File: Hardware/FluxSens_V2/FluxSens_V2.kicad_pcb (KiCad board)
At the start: 2 copper layers, 35 parts, among them J1 Conn_01x08, U1 HMC1051Z, U2 RC4558, U3 MAX662ACSA+

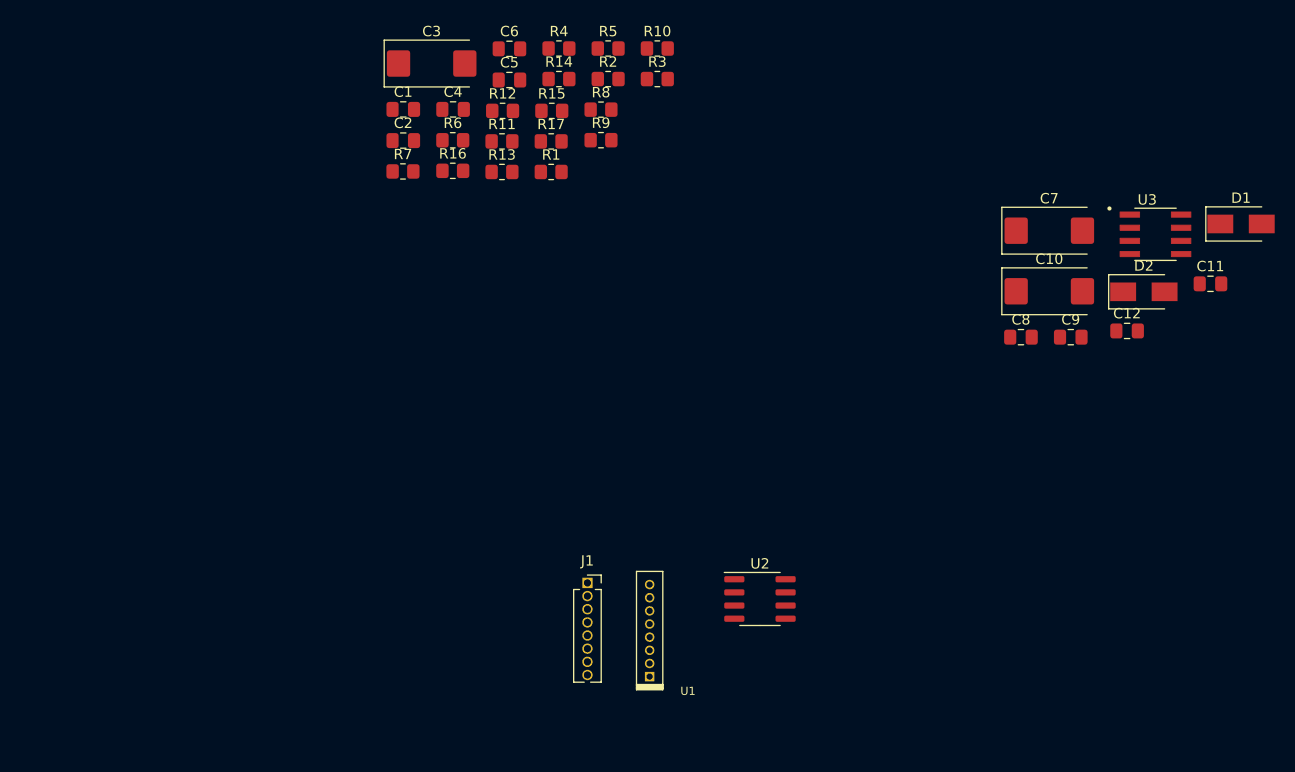
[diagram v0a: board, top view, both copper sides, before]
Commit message: finished the V2 board layout
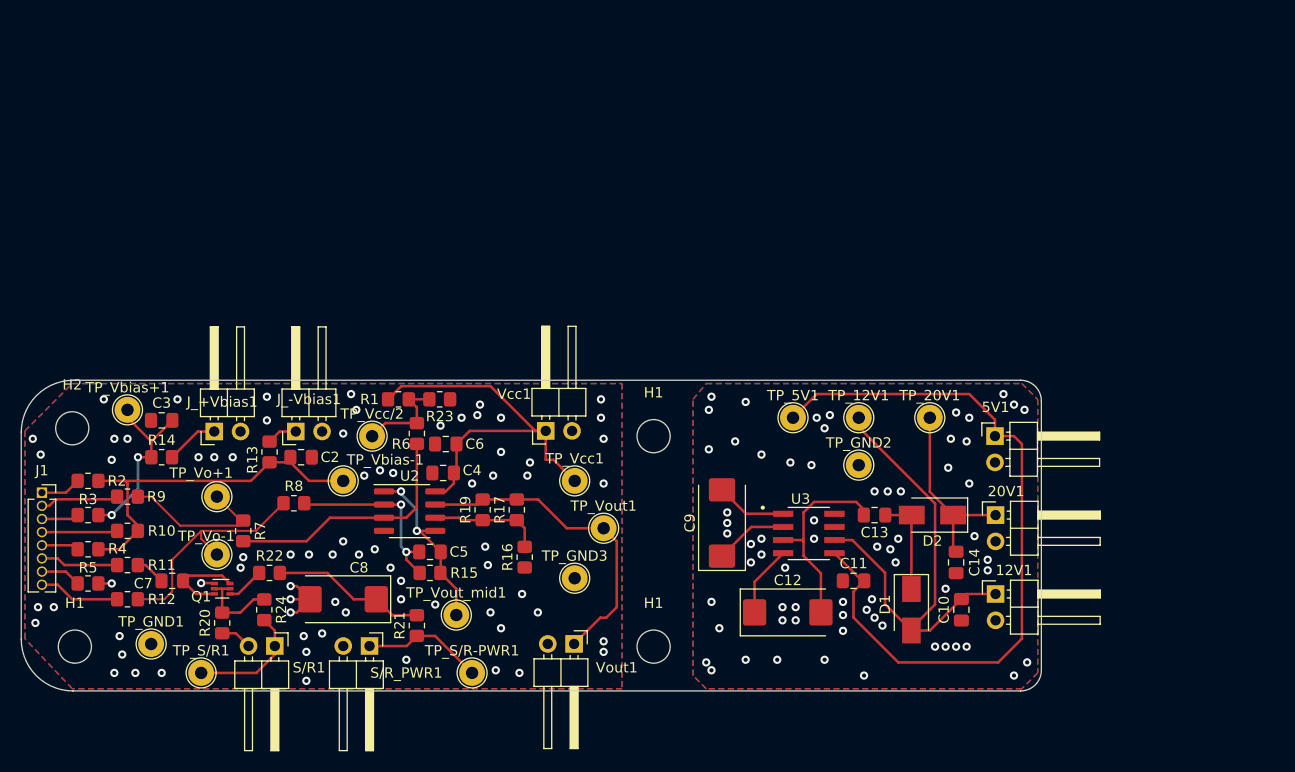
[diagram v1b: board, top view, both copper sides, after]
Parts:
- removed C1: 100nf, Capacitor_SMD:C_0805_2012Metric_Pad1.18x1.45mm_HandSolder
- removed U1: HMC1051Z, MyLib:HMC1051Z3
- added 12V1: Conn_01x02, Connector_PinHeader_2.54mm:PinHeader_1x02_P2.54mm_Horizontal, F.Cu at (195.6, 104.1)
- added 20V1: Conn_01x02, Connector_PinHeader_2.54mm:PinHeader_1x02_P2.54mm_Horizontal, F.Cu at (195.6, 96.5)
- added 5V1: Conn_01x02, Connector_PinHeader_2.54mm:PinHeader_1x02_P2.54mm_Horizontal, F.Cu at (195.5, 88.9)
- added C13: 100nf, Capacitor_SMD:C_0805_2012Metric_Pad1.18x1.45mm_HandSolder, F.Cu at (183.9, 96.5)
- added C14: 100nf, Capacitor_SMD:C_0805_2012Metric_Pad1.18x1.45mm_HandSolder, F.Cu at (191.8, 101.1)
- added H1: MountingHole, MountingHole:MountingHole_3.2mm_M3, F.Cu at (106.7, 109.2)
- added H1: MountingHole, MountingHole:MountingHole_3.2mm_M3, F.Cu at (162.6, 109.2)
- added H1: MountingHole, MountingHole:MountingHole_3.2mm_M3, F.Cu at (162.6, 88.9)
- added H2: MountingHole, MountingHole:MountingHole_3.2mm_M3, F.Cu at (106.4, 88.1)
- added J_+Vbias1: Conn_01x02, Connector_PinHeader_2.54mm:PinHeader_1x02_P2.54mm_Horizontal, F.Cu at (120.1, 88.4)
- added J_-Vbias1: Conn_01x02, Connector_PinHeader_2.54mm:PinHeader_1x02_P2.54mm_Horizontal, F.Cu at (128.0, 88.4)
- added Q1: BSD235C, Package_TO_SOT_SMD:SOT-563, F.Cu at (120.9, 103.6)
- added R19: Rth, Resistor_SMD:R_0805_2012Metric_Pad1.20x1.40mm_HandSolder, F.Cu at (146.1, 96.0)
- added R20: 4k7, Resistor_SMD:R_0805_2012Metric_Pad1.20x1.40mm_HandSolder, F.Cu at (120.9, 106.9)
- added R21: 180R, Resistor_SMD:R_0805_2012Metric_Pad1.20x1.40mm_HandSolder, F.Cu at (139.7, 107.2)
- added R22: 0R, Resistor_SMD:R_0805_2012Metric_Pad1.20x1.40mm_HandSolder, F.Cu at (125.5, 102.1)
- added R23: 10k, Resistor_SMD:R_0805_2012Metric_Pad1.20x1.40mm_HandSolder, F.Cu at (141.9, 85.3)
- added R24: 0R, Resistor_SMD:R_0805_2012Metric_Pad1.20x1.40mm_HandSolder, F.Cu at (125.0, 105.7)
- added S/R1: Conn_01x02, Connector_PinHeader_2.54mm:PinHeader_1x02_P2.54mm_Horizontal, F.Cu at (126.0, 109.2)
- added S/R_PWR1: Conn_01x02, Connector_PinHeader_2.54mm:PinHeader_1x02_P2.54mm_Horizontal, F.Cu at (135.1, 109.2)
- added TP_12V1: TestPoint, TestPoint:TestPoint_THTPad_D2.5mm_Drill1.2mm, F.Cu at (182.4, 87.1)
- added TP_20V1: TestPoint, TestPoint:TestPoint_THTPad_D2.5mm_Drill1.2mm, F.Cu at (189.2, 87.1)
- added TP_5V1: TestPoint, TestPoint:TestPoint_THTPad_D2.5mm_Drill1.2mm, F.Cu at (176.0, 87.1)
- added TP_GND1: TestPoint, TestPoint:TestPoint_THTPad_D2.5mm_Drill1.2mm, F.Cu at (114.0, 109.0)
- added TP_GND2: TestPoint, TestPoint:TestPoint_THTPad_D2.5mm_Drill1.2mm, F.Cu at (182.4, 91.7)
- added TP_GND3: TestPoint, TestPoint:TestPoint_THTPad_D2.5mm_Drill1.2mm, F.Cu at (154.9, 102.6)
- added TP_S/R-PWR1: TestPoint, TestPoint:TestPoint_THTPad_D2.5mm_Drill1.2mm, F.Cu at (145.0, 111.8)
- added TP_S/R1: TestPoint, TestPoint:TestPoint_THTPad_D2.5mm_Drill1.2mm, F.Cu at (118.9, 111.8)
- added TP_Vbias+1: TestPoint, TestPoint:TestPoint_THTPad_D2.5mm_Drill1.2mm, F.Cu at (111.8, 86.4)
- added TP_Vbias-1: TestPoint, TestPoint:TestPoint_THTPad_D2.5mm_Drill1.2mm, F.Cu at (132.6, 93.2)
- added TP_Vcc/2: TestPoint, TestPoint:TestPoint_THTPad_D2.5mm_Drill1.2mm, F.Cu at (135.4, 88.9)
- added TP_Vcc1: TestPoint, TestPoint:TestPoint_THTPad_D2.5mm_Drill1.2mm, F.Cu at (154.9, 93.2)
- added TP_Vo+1: TestPoint, TestPoint:TestPoint_THTPad_D2.5mm_Drill1.2mm, F.Cu at (120.4, 94.7)
- added TP_Vo-1: TestPoint, TestPoint:TestPoint_THTPad_D2.5mm_Drill1.2mm, F.Cu at (120.4, 100.3)
- added TP_Vout1: TestPoint, TestPoint:TestPoint_THTPad_D2.5mm_Drill1.2mm, F.Cu at (157.7, 97.8)
- added TP_Vout_mid1: TestPoint, TestPoint:TestPoint_THTPad_D2.5mm_Drill1.2mm, F.Cu at (143.5, 106.2)
- added Vcc1: Conn_01x02, Connector_PinHeader_2.54mm:PinHeader_1x02_P2.54mm_Horizontal, F.Cu at (152.1, 88.4)
- added Vout1: Conn_01x02, Connector_PinHeader_2.54mm:PinHeader_1x02_P2.54mm_Horizontal, F.Cu at (154.9, 109.0)
- C10: value C_Polarized_Small -> 100nf; footprint Capacitor_Tantalum_SMD:CP_EIA-7343-31_Kemet-D_Pad2.25x2.55mm_HandSolder -> Capacitor_SMD:C_0805_2012Metric_Pad1.18x1.45mm_HandSolder
- C11: value 100nf -> 2uf
- C12, C8: value 100nf -> C_Polarized_Small; footprint Capacitor_SMD:C_0805_2012Metric_Pad1.18x1.45mm_HandSolder -> Capacitor_Tantalum_SMD:CP_EIA-7343-31_Kemet-D_Pad2.25x2.55mm_HandSolder
- C2: value C_Small -> 1u
- C3: value C_Polarized_Small -> 1u; footprint Capacitor_Tantalum_SMD:CP_EIA-7343-31_Kemet-D_Pad2.25x2.55mm_HandSolder -> Capacitor_SMD:C_0805_2012Metric_Pad1.18x1.45mm_HandSolder
- C5: value C_Small -> 100nf
- C7: value C_Polarized_Small -> C_Small; footprint Capacitor_Tantalum_SMD:CP_EIA-7343-31_Kemet-D_Pad2.25x2.55mm_HandSolder -> Capacitor_SMD:C_0805_2012Metric_Pad1.18x1.45mm_HandSolder
- C9: value 2uf -> C_Polarized_Small; footprint Capacitor_SMD:C_0805_2012Metric_Pad1.18x1.45mm_HandSolder -> Capacitor_Tantalum_SMD:CP_EIA-7343-31_Kemet-D_Pad2.25x2.55mm_HandSolder
- R1: value R_Small -> 10k
- R12, R5: value 500k -> R_Small
- R13: value Rb -> 4R
- R14: value R_Small -> 4R
- R15: value Ra -> 500k
- R16: value Rth -> Rb
- R17: value R_Small -> Ra
- R6: value 5k -> 500k
- R8: value R_Small -> 5k
- moved C7 91.2 mm to (116.1, 102.9)
- moved R5 72.0 mm to (108.0, 103.1)
- moved C8 70.2 mm to (132.6, 104.6), turned to 180 degrees
- moved R3 69.2 mm to (108.0, 96.5)
- moved R10 69.2 mm to (111.8, 98.0)
- moved R4 66.4 mm to (108.0, 99.8)
- moved R2 63.5 mm to (108.0, 93.2)
- moved R12 59.5 mm to (111.8, 104.6)
- moved R9 57.2 mm to (111.8, 94.7)
- moved R11 54.6 mm to (111.8, 101.3)
- moved J1 53.4 mm to (103.5, 94.4)
- moved R14 53.0 mm to (115.1, 90.9)
- moved D1 49.0 mm to (187.5, 105.7), turned to -90 degrees
- moved R8 48.2 mm to (127.8, 95.4)
- moved C5 46.2 mm to (141.0, 100.1)
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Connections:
- C10 pad 1: Net-(C10-Pad1) -> GND2
- C10 pad 2: Net-(C10-Pad2) -> /+12V
- C11 pad 1: Net-(C11-Pad1) -> GND2
- C11 pad 2: Net-(C10-Pad2) -> /5V
- C12 pad 1: GND -> Net-(C12-Pad1)
- C12 pad 2: /20V -> Net-(C12-Pad2)
- C2 pad 1: unconnected-(C2-Pad1) -> GND
- C2 pad 2: unconnected-(C2-Pad2) -> /-Vbias
- C3 pad 1: Net-(C3-Pad1) -> GND
- C3 pad 2: GND -> /+Vbias
- C4 pad 1: unconnected-(C4-Pad1) -> GND
- C4 pad 2: unconnected-(C4-Pad2) -> /Vcc
- C5 pad 1: GND -> Net-(C5-Pad1)
- C5 pad 2: /Vcc -> Net-(C5-Pad2)
- C7 pad 1: Net-(C7-Pad1) -> /S/R+
- C7 pad 2: Net-(C7-Pad2) -> Net-(Q1-Pad3)
- C8 pad 1: GND -> Net-(C8-Pad1)
- C8 pad 2: Net-(C8-Pad2) -> GND
- C9 pad 1: GND -> Net-(C9-Pad1)
- C9 pad 2: /+5V -> Net-(C9-Pad2)
- D1 pad 1: Net-(C11-Pad1) -> Net-(C13-Pad1)
- D1 pad 2: Net-(C8-Pad2) -> /+12V
- D2 pad 2: Net-(C11-Pad1) -> Net-(C13-Pad1)
- R1 pad 1: Net-(J1-Pad1) -> /Vcc/2
- R1 pad 2: GND -> /Vcc
- R10 pad 1: Net-(J1-Pad6) -> Net-(J1-Pad4)
- R10 pad 2: /S/R+ -> /-Vbias
- R11 pad 1: Net-(J1-Pad8) -> Net-(J1-Pad6)
- R11 pad 2: /Vo- -> /S/R+
- R12 pad 1: Net-(U2-Pad2) -> Net-(J1-Pad8)
- R12 pad 2: Net-(U2-Pad1) -> /Vo-
- R13 pad 1: GND -> /-Vbias
- R13 pad 2: Net-(U2-Pad6) -> Net-(J_-Vbias1-Pad1)
- R14 pad 1: /Vcc -> /+Vbias
- R14 pad 2: Net-(C3-Pad1) -> Net-(J_+Vbias1-Pad1)
- R15 pad 1: Net-(U2-Pad6) -> Net-(C5-Pad1)
- R15 pad 2: /Vo -> Net-(C5-Pad2)
- R16 pad 1: Net-(U2-Pad6) -> GND
- R16 pad 2: /Vo -> Net-(R16-Pad2)
- R17 pad 1: unconnected-(R17-Pad1) -> Net-(R16-Pad2)
- R17 pad 2: unconnected-(R17-Pad2) -> /Vo
- R2 pad 1: Net-(J1-Pad3) -> Net-(J1-Pad1)
- R2 pad 2: /Vcc -> /-Vbias
- R3 pad 1: Net-(J1-Pad5) -> Net-(J1-Pad3)
- R3 pad 2: GND -> /+Vbias
- R4 pad 1: Net-(J1-Pad7) -> Net-(J1-Pad5)
- R4 pad 2: /S/R- -> /-Vbias
- R5 pad 1: /Vcc/2 -> Net-(J1-Pad7)
- R5 pad 2: Net-(U2-Pad3) -> GND
- R6 pad 1: /Vo+ -> /Vcc/2
- R6 pad 2: Net-(U2-Pad3) -> Net-(R6-Pad2)
- R7 pad 1: /Vo- -> /Vo+
- R7 pad 2: Net-(U2-Pad2) -> Net-(R6-Pad2)
- R8 pad 1: Net-(J1-Pad2) -> /Vo-
- R8 pad 2: /Vo+ -> Net-(C5-Pad1)
- R9 pad 1: Net-(J1-Pad4) -> Net-(J1-Pad2)
- R9 pad 2: GND -> /Vo+
- U2 pad 1: Net-(U2-Pad1) -> Net-(C5-Pad2)
- U2 pad 2: Net-(U2-Pad2) -> Net-(C5-Pad1)
- U2 pad 3: Net-(U2-Pad3) -> Net-(R6-Pad2)
- U2 pad 5: Net-(U2-Pad1) -> Net-(C5-Pad2)
- U2 pad 6: Net-(U2-Pad6) -> Net-(R16-Pad2)
- U3 pad 1: Net-(C7-Pad2) -> Net-(C9-Pad2)
- U3 pad 2: Net-(C7-Pad1) -> Net-(C9-Pad1)
- U3 pad 3: Net-(C10-Pad2) -> Net-(C12-Pad2)
- U3 pad 4: Net-(C10-Pad1) -> Net-(C12-Pad1)
- U3 pad 5: /+5V -> /5V
- U3 pad 6: Net-(C8-Pad2) -> /+12V
- U3 pad 7: GND -> GND2
- U3 pad 8: GND -> GND2
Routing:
- net /5V: track 0.00 -> 71.8 mm
- net /+12V: track 0.00 -> 46.9 mm
- net /Vcc: track 0.00 -> 39.1 mm
- net /-Vbias: track 0.00 -> 35.7 mm
- net /Vo: track 0.00 -> 31.3 mm
- net Net-(R6-Pad2): track 0.00 -> 24.2 mm
- net /Vo-: track 0.00 -> 22.6 mm
- net Net-(C12-Pad2): track 0.00 -> 19.4 mm
- net /20V: track 0.00 -> 18.1 mm
- net Net-(C5-Pad1): track 0.00 -> 18.0 mm, vias 0 -> 2
- net Net-(C5-Pad2): track 0.00 -> 17.8 mm, vias 0 -> 2
- net /+Vbias: track 0.00 -> 17.6 mm, vias 0 -> 2
- net /Vo+: track 0.00 -> 15.0 mm
- net Net-(C8-Pad1): track 0.00 -> 14.9 mm
- net GND: track 0.00 -> 12.3 mm, vias 0 -> 74
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- added copper zone on B.Cu, net GND
- added copper zone on F.Cu, net GND
- added copper zone on B.Cu, net GND2
- added copper zone on F.Cu, net GND2
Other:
- board outline added: 98.5 x 30 mm

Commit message: update
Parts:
- C10, C13, C14, C5: value 100nf -> 100nF
- C2, C3: value 1u -> 1uF
- C4: value C_Small -> 1uF
- C6, C7: value C_Small -> 0.1uF
- R10, R11, R12, R2, R3, R4, R5, R9: value R_Small -> 0R
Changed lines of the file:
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@@
   (net 11 "Net-(R6-Pad2)")
   (net 12 "Net-(J_-Vbias1-Pad1)")
-  (net 13 "Net-(Q1-Pad3)")
+  (net 13 "Net-(C7-Pad2)")
   (net 14 "/-Vbias")
   (net 15 "/+Vbias")
@@
   (net 34 "/Vo-")
   (net 35 "Net-(R16-Pad2)")
-  (net 36 "Net-(S/R_PWR1-Pad1)")
-  (net 37 "Net-(S/R1-Pad1)")
+  (net 36 "Net-(R21-Pad1)")
+  (net 37 "Net-(R24-Pad2)")
   (net 38 "GND2")
   (footprint "Connector_PinHeader_2.54mm:PinHeader_1x02_P2.54mm_Horizontal" (layer "F.Cu")
@@
     (fp_line (start 1.5 -0.635) (end 2.135 -1.27) (layer "F.Fab") (width 0.1))
     (pad "1" thru_hole rect (at 0 0 270) (size 1.7 1.7) (drill 1) (layers *.Cu *.Mask)
-      (net 37 "Net-(S/R1-Pad1)") (pinfunction "Pin_1") (pintype "passive"))
+      (net 37 "Net-(R24-Pad2)") (pinfunction "Pin_1") (pintype "passive"))
     (pad "2" thru_hole oval (at 0 2.54 270) (size 1.7 1.7) (drill 1) (layers *.Cu *.Mask)
       (net 1 "GND") (pinfunction "Pin_2") (pintype "passive"))
@@
       (effects (font (size 1 1) (thickness 0.15)))
     )
-    (fp_text value "C_Small" (at 0 1.68) (layer "F.Fab")
+    (fp_text value "0.1uF" (at 0 1.68) (layer "F.Fab")
       (effects (font (size 1 1) (thickness 0.15)))
     )
@@
       (net 19 "/S{slash}R+") (pintype "passive"))
     (pad "2" smd roundrect (at 1.0375 0) (size 1.175 1.45) (layers "F.Cu" "F.Paste" "F.Mask") (roundrect_rratio 0.212766)
-      (net 13 "Net-(Q1-Pad3)") (pintype "passive"))
+      (net 13 "Net-(C7-Pad2)") (pintype "passive"))
     (model "${KICAD6_3DMODEL_DIR}/Capacitor_SMD.3dshapes/C_0805_2012Metric.wrl"
       (offset (xyz 0 0 0))
@@
       (effects (font (size 1 1) (thickness 0.15)))
     )
-    (fp_text value "100nf" (at 0 1.68) (layer "F.Fab")
+    (fp_text value "100nF" (at 0 1.68) (layer "F.Fab")
       (effects (font (size 1 1) (thickness 0.15)))
     )
@@
       (effects (font (size 1 1) (thickness 0.15)))
     )
-    (fp_text value "C_Small" (at 0 1.68) (layer "F.Fab")
+    (fp_text value "1uF" (at 0 1.68) (layer "F.Fab")
       (effects (font (size 1 1) (thickness 0.15)))
     )
@@
       (effects (font (size 1 1) (thickness 0.15)))
     )
-    (fp_text value "R_Small" (at 0 1.65) (layer "F.Fab")
+    (fp_text value "0R" (at 0 1.65) (layer "F.Fab")
       (effects (font (size 1 1) (thickness 0.15)))
     )
@@
       (effects (font (size 1 1) (thickness 0.15)))
     )
-    (fp_text value "1u" (at 0 1.68) (layer "F.Fab")
+    (fp_text value "1uF" (at 0 1.68) (layer "F.Fab")
       (effects (font (size 1 1) (thickness 0.15)))
     )
@@
       (effects (font (size 1 1) (thickness 0.15)))
     )
-    (fp_text value "R_Small" (at 0 1.65) (layer "F.Fab")
+    (fp_text value "0R" (at 0 1.65) (layer "F.Fab")
       (effects (font (size 1 1) (thickness 0.15)))
     )
@@
       (effects (font (size 1 1) (thickness 0.15)))
     )
-    (fp_text value "100nf" (at 0 1.68 90) (layer "F.Fab")
+    (fp_text value "100nF" (at 0 1.68 90) (layer "F.Fab")
       (effects (font (size 1 1) (thickness 0.15)))
     )
@@
       (effects (font (size 1 1) (thickness 0.15)))
     )
-    (fp_text value "1u" (at 0 1.68) (layer "F.Fab")
+    (fp_text value "1uF" (at 0 1.68) (layer "F.Fab")
       (effects (font (size 1 1) (thickness 0.15)))
     )
@@
     (fp_circle (center 0 0) (end 1.75 0) (layer "F.CrtYd") (width 0.05) (fill none))
     (pad "1" thru_hole circle (at 0 0) (size 2.5 2.5) (drill 1.2) (layers *.Cu *.Mask)
-      (net 37 "Net-(S/R1-Pad1)") (pinfunction "1") (pintype "passive"))
+      (net 37 "Net-(R24-Pad2)") (pinfunction "1") (pintype "passive"))
   )
   (footprint "Resistor_SMD:R_0805_2012Metric_Pad1.20x1.40mm_HandSolder" (layer "F.Cu")
@@
       (effects (font (size 1 1) (thickness 0.15)))
     )
-    (fp_text value "R_Small" (at 0 1.65) (layer "F.Fab")
+    (fp_text value "0R" (at 0 1.65) (layer "F.Fab")
       (effects (font (size 1 1) (thickness 0.15)))
     )
@@
       (effects (font (size 1 1) (thickness 0.15)))
     )
-    (fp_text value "C_Small" (at 0 1.68) (layer "F.Fab")
+    (fp_text value "0.1uF" (at 0 1.68) (layer "F.Fab")
       (effects (font (size 1 1) (thickness 0.15)))
     )
@@
     (fp_line (start -1 0.625) (end -1 -0.625) (layer "F.Fab") (width 0.1))
     (pad "1" smd roundrect (at -1 0 90) (size 1.2 1.4) (layers "F.Cu" "F.Paste" "F.Mask") (roundrect_rratio 0.208333)
-      (net 36 "Net-(S/R_PWR1-Pad1)") (pintype "passive"))
+      (net 36 "Net-(R21-Pad1)") (pintype "passive"))
     (pad "2" smd roundrect (at 1 0 90) (size 1.2 1.4) (layers "F.Cu" "F.Paste" "F.Mask") (roundrect_rratio 0.208333)
       (net 20 "Net-(C8-Pad1)") (pintype "passive"))
@@
       (effects (font (size 1 1) (thickness 0.15)))
     )
-    (fp_text value "R_Small" (at 0 1.65) (layer "F.Fab")
+    (fp_text value "0R" (at 0 1.65) (layer "F.Fab")
       (effects (font (size 1 1) (thickness 0.15)))
     )
@@
       (net 29 "/S{slash}R") (pinfunction "GN") (pintype "input"))
     (pad "3" smd rect (at -0.75 0.5) (size 0.7 0.34) (layers "F.Cu" "F.Paste" "F.Mask")
-      (net 13 "Net-(Q1-Pad3)") (pinfunction "DP") (pintype "passive"))
+      (net 13 "Net-(C7-Pad2)") (pinfunction "DP") (pintype "passive"))
     (pad "4" smd rect (at 0.75 0.5) (size 0.7 0.34) (layers "F.Cu" "F.Paste" "F.Mask")
       (net 31 "Net-(Q1-Pad4)") (pinfunction "SP") (pintype "passive"))
@@
       (net 29 "/S{slash}R") (pinfunction "GP") (pintype "input"))
     (pad "6" smd rect (at 0.75 -0.5) (size 0.7 0.34) (layers "F.Cu" "F.Paste" "F.Mask")
-      (net 13 "Net-(Q1-Pad3)") (pinfunction "DN") (pintype "passive"))
+      (net 13 "Net-(C7-Pad2)") (pinfunction "DN") (pintype "passive"))
     (model "${KICAD6_3DMODEL_DIR}/Package_TO_SOT_SMD.3dshapes/SOT-563.wrl"
       (offset (xyz 0 0 0))
@@
     (fp_circle (center 0 0) (end 1.75 0) (layer "F.CrtYd") (width 0.05) (fill none))
     (pad "1" thru_hole circle (at 0 0) (size 2.5 2.5) (drill 1.2) (layers *.Cu *.Mask)
-      (net 36 "Net-(S/R_PWR1-Pad1)") (pinfunction "1") (pintype "passive"))
+      (net 36 "Net-(R21-Pad1)") (pinfunction "1") (pintype "passive"))
   )
   (footprint "Capacitor_SMD:C_0805_2012Metric_Pad1.18x1.45mm_HandSolder" (layer "F.Cu")
@@
       (effects (font (size 1 1) (thickness 0.15)))
     )
-    (fp_text value "100nf" (at 0 1.68 90) (layer "F.Fab")
+    (fp_text value "100nF" (at 0 1.68 90) (layer "F.Fab")
       (effects (font (size 1 1) (thickness 0.15)))
     )
@@
       (effects (font (size 1 1) (thickness 0.15)))
     )
-    (fp_text value "R_Small" (at 0 1.65) (layer "F.Fab")
+    (fp_text value "0R" (at 0 1.65) (layer "F.Fab")
       (effects (font (size 1 1) (thickness 0.15)))
     )
@@
       (effects (font (size 1 1) (thickness 0.15)))
     )
-    (fp_text value "100nf" (at 0 1.68) (layer "F.Fab")
+    (fp_text value "100nF" (at 0 1.68) (layer "F.Fab")
       (effects (font (size 1 1) (thickness 0.15)))
     )
@@
       (effects (font (size 1 1) (thickness 0.15)))
     )
-    (fp_text value "R_Small" (at 0 1.65) (layer "F.Fab")
+    (fp_text value "0R" (at 0 1.65) (layer "F.Fab")
       (effects (font (size 1 1) (thickness 0.15)))
     )
@@
       (effects (font (size 1 1) (thickness 0.15)))
     )
-    (fp_text value "R_Small" (at 0 1.65) (layer "F.Fab")
+    (fp_text value "0R" (at 0 1.65) (layer "F.Fab")
       (effects (font (size 1 1) (thickness 0.15)))
     )
@@
       (effects (font (size 1 1) (thickness 0.15)))
     )
-    (fp_text value "R_Small" (at 0 1.65) (layer "F.Fab")
+    (fp_text value "0R" (at 0 1.65) (layer "F.Fab")
       (effects (font (size 1 1) (thickness 0.15)))
     )
@@
     (fp_line (start 4.04 2.86) (end 10.04 2.86) (layer "F.Fab") (width 0.1))
     (pad "1" thru_hole rect (at 0 0 270) (size 1.7 1.7) (drill 1) (layers *.Cu *.Mask)
-      (net 36 "Net-(S/R_PWR1-Pad1)") (pinfunction "Pin_1") (pintype "passive"))
+      (net 36 "Net-(R21-Pad1)") (pinfunction "Pin_1") (pintype "passive"))
     (pad "2" thru_hole oval (at 0 2.54 270) (size 1.7 1.7) (drill 1) (layers *.Cu *.Mask)
       (net 1 "GND") (pinfunction "Pin_2") (pintype "passive"))
@@
       (net 29 "/S{slash}R") (pintype "passive"))
     (pad "2" smd roundrect (at 1 0 270) (size 1.2 1.4) (layers "F.Cu" "F.Paste" "F.Mask") (roundrect_rratio 0.208333)
-      (net 37 "Net-(S/R1-Pad1)") (pintype "passive"))
+      (net 37 "Net-(R24-Pad2)") (pintype "passive"))
     (model "${KICAD6_3DMODEL_DIR}/Resistor_SMD.3dshapes/R_0805_2012Metric.wrl"
       (offset (xyz 0 0 0))
